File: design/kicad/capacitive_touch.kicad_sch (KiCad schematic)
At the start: 23 parts, among them J15 Conn_01x12_Socket, J5 Conn_01x12_Socket, J6 Conn_01x12_Socket, J7 Conn_01x12_Socket, U10 MPR121QR2, U4 MPR121QR2, U5 MPR121QR2, U6 MPR121QR2

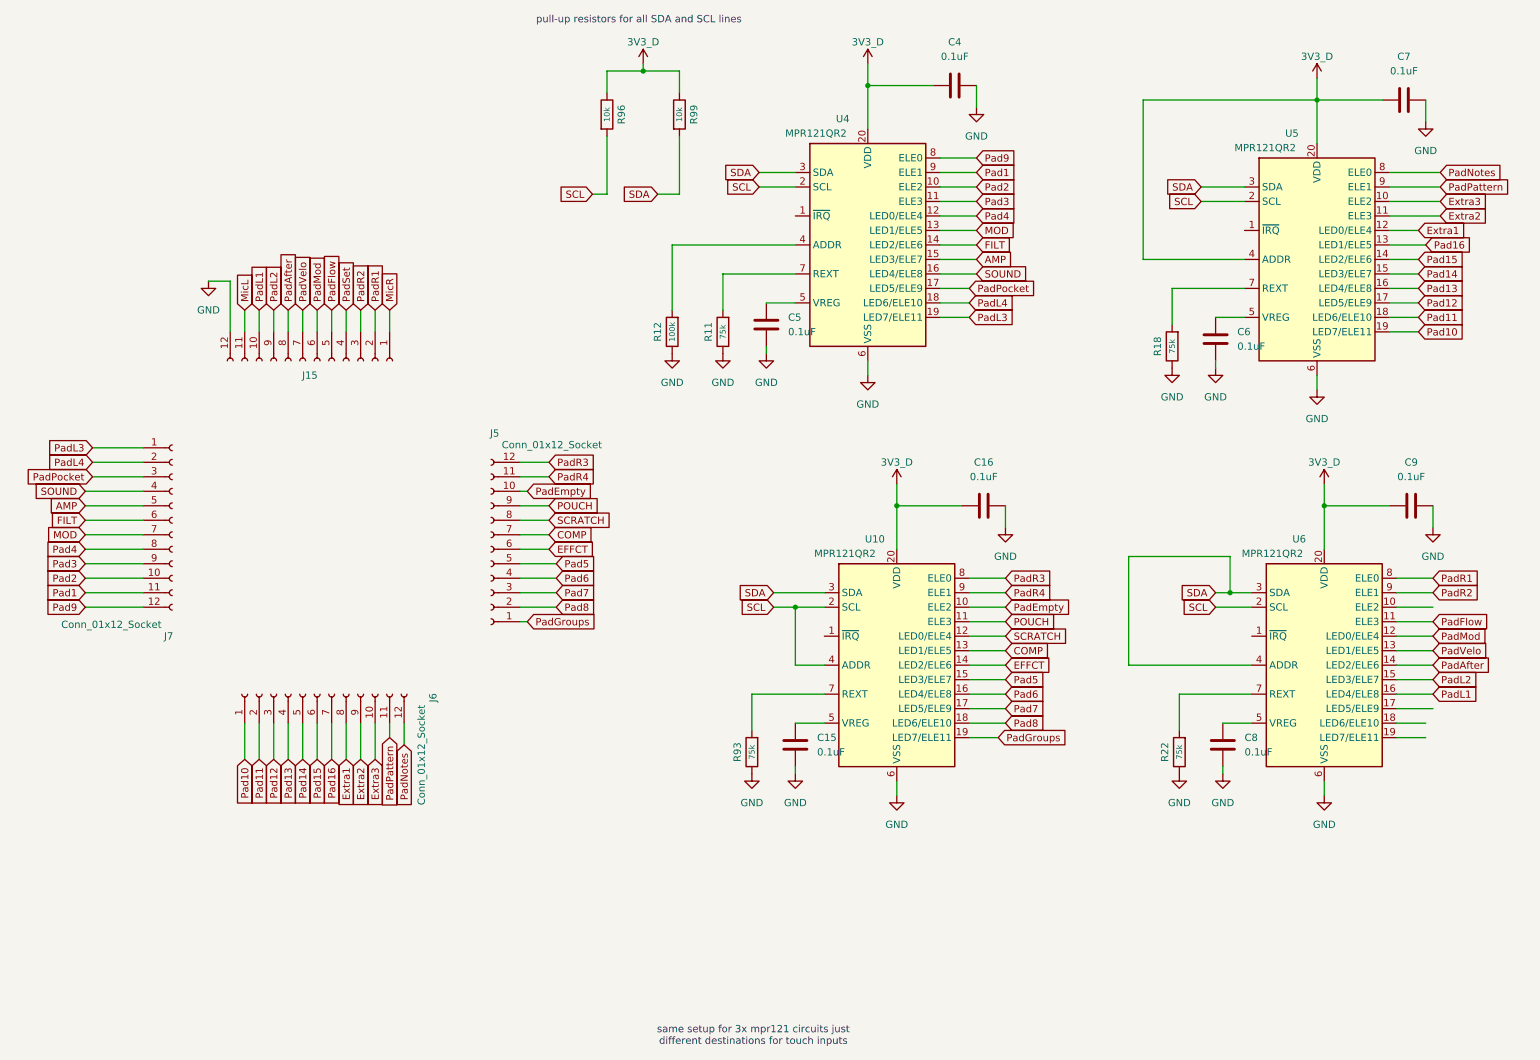
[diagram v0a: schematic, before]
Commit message: last commit before refactor repo: kicad mostly
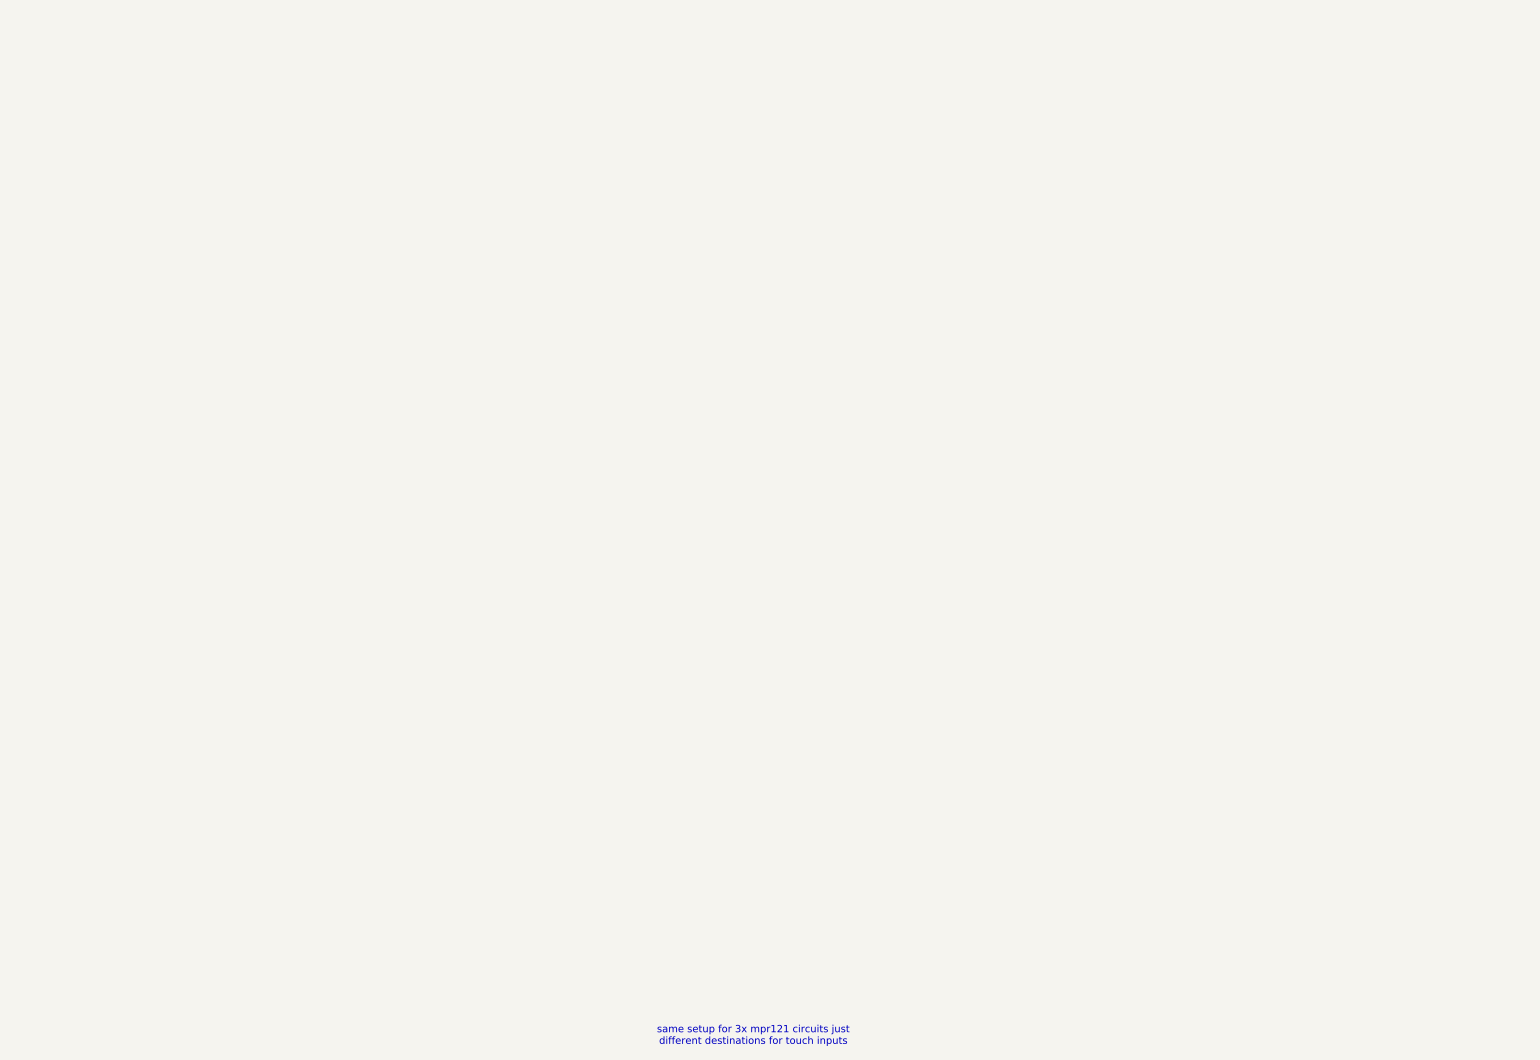
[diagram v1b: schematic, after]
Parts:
- removed C15, C16, C4, C5, C6, C7, C8, C9: 0.1uF, Capacitor_SMD:C_0402_1005Metric, symbol Device:C
- removed J15, J5, J6, J7: Conn_01x12_Socket, Connector_PinSocket_1.27mm:PinSocket_1x12_P1.27mm_Vertical, symbol Connector:Conn_01x12_Socket
- removed R11, R18, R22, R93: 75k, Resistor_SMD:R_0603_1608Metric, symbol Device:R
- removed R12: 100k, Resistor_SMD:R_0402_1005Metric, symbol Device:R
- removed R96, R99: 10k, Resistor_SMD:R_0603_1608Metric, symbol Device:R
- removed U10, U4, U5, U6: MPR121QR2, Package_DFN_QFN:UQFN-20_3x3mm_P0.4mm, symbol Sensor_Touch:MPR121QR2
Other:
- note removed: "pull-up resistors for all SDA and SCL lines"
